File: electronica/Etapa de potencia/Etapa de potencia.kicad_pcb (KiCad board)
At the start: 2 copper layers, 70 x 45 mm, 23 parts, among them J1 Bornera Resorte, J2 Bornera Resorte, J3 Bornera Resorte, J4 Bornera 4 pines, J5 Header, Q1 MMBT2222, Q2 MMBT2222, Q3 MMBT2222, U1 ATmega328-PU, U2 ULN2003, U3 ULN2003, U4 MOC3031M, Y1 Crystal

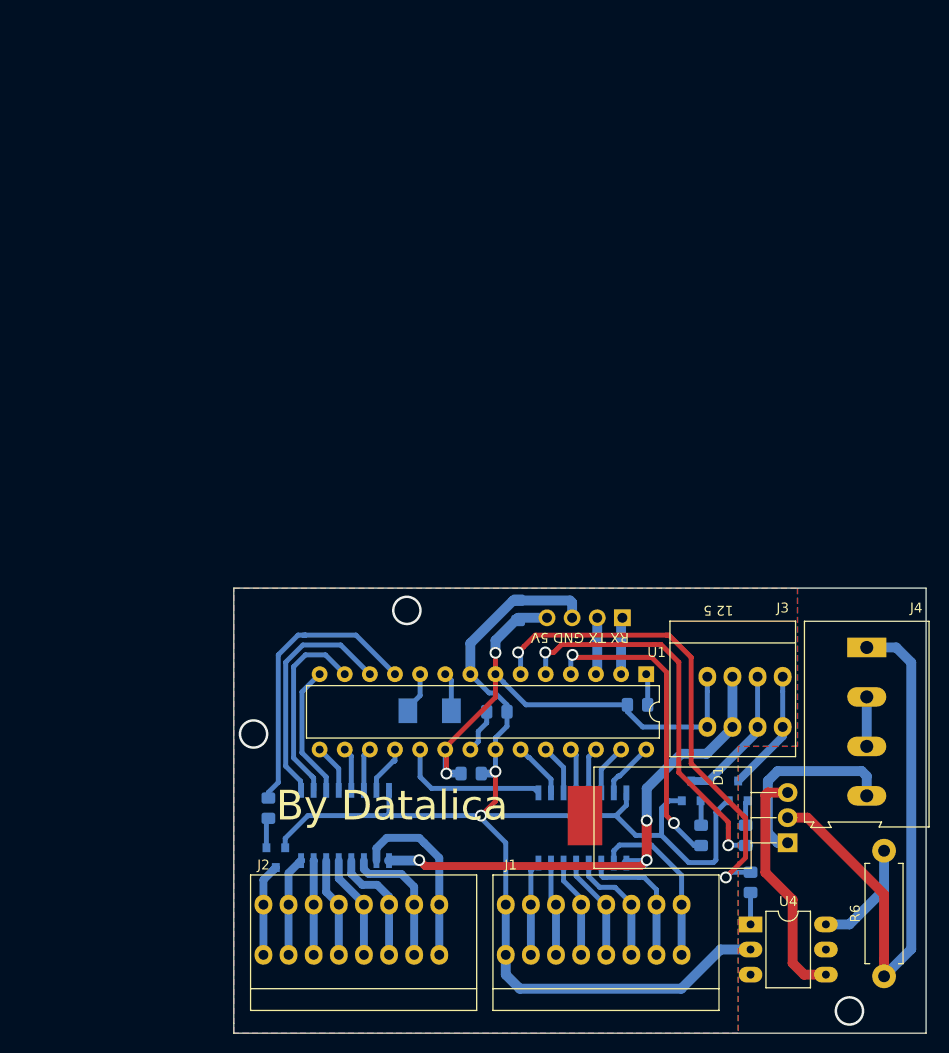
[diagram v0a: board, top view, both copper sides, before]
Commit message: ending first pcb
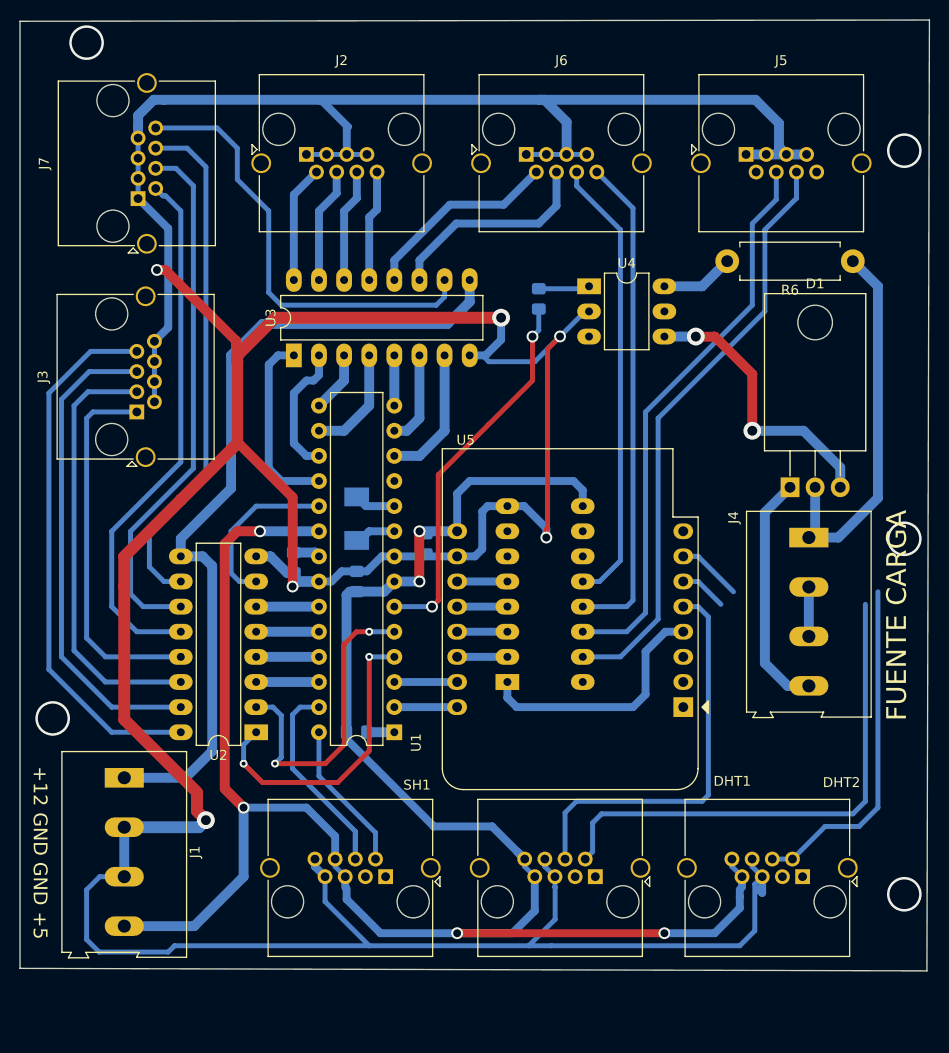
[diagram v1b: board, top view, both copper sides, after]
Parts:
- removed Q1, Q2, Q3: MMBT2222, Package_TO_SOT_SMD:SOT-23
- removed R3, R4, R5: 1K, Resistor_SMD:R_0805_2012Metric_Pad1.15x1.40mm_HandSolder
- added DHT1: RJ45, Connector_RJ:RJ45_Amphenol_RJHSE5380, F.Cu at (122.6, 130.2)
- added DHT2: RJ45, Connector_RJ:RJ45_Amphenol_RJHSE5380, F.Cu at (143.5, 130.2)
- added J6: RJ45, Connector_RJ:RJ45_Amphenol_RJHSE5380, F.Cu at (115.6, 57.1)
- added J7: RJ45, Connector_RJ:RJ45_Amphenol_RJHSE5380, F.Cu at (76.3, 61.6)
- added SH1: RJ45, Connector_RJ:RJ45_Amphenol_RJHSE5380, F.Cu at (101.3, 130.2)
- added U5: WeMos_D1_mini, Module:WEMOS_D1_mini_light, F.Cu at (131.4, 113.0)
- added U6: ULN2002A, Package_DIP:DIP-16_W7.62mm_LongPads, B.Cu at (113.7, 110.5)
- J1: value Bornera Resorte -> Bornera 4 pines; footprint potenciaFootprints:BorneraKF141R_8Pins -> TerminalBlock:TerminalBlock_Altech_AK300-4_P5.00mm
- J2: value Bornera Resorte -> RJ45; footprint potenciaFootprints:BorneraKF141R_8Pins -> Connector_RJ:RJ45_Amphenol_RJHSE5380
- J3: value Bornera Resorte -> RJ45; footprint potenciaFootprints:BorneraKF141R_4Pins -> Connector_RJ:RJ45_Amphenol_RJHSE5380
- J5: value Header -> RJ45; footprint Connector_PinHeader_2.54mm:PinHeader_1x04_P2.54mm_Vertical -> Connector_RJ:RJ45_Amphenol_RJHSE5380; moved to F.Cu
- U2, U3: footprint Package_SO:SOIC-16W_5.3x10.2mm_P1.27mm -> Package_DIP:DIP-16_W7.62mm_LongPads; moved to F.Cu
- moved J3 74.0 mm to (76.2, 83.2), turned to 90 degrees
- moved J2 73.0 mm to (93.3, 57.1)
- moved R6 72.4 mm to (148.6, 67.9), turned to 180 degrees
- moved U4 66.5 mm to (121.9, 70.5)
- moved R2 62.8 mm to (116.8, 71.8), turned to 270 degrees
- moved J5 48.5 mm to (137.8, 57.1), turned to 0 degrees
- moved U3 47.8 mm to (92.1, 77.5), turned to 90 degrees
- moved J1 39.8 mm to (74.9, 120.2), turned to 270 degrees
- moved D1 35.9 mm to (142.2, 90.8), turned to 0 degrees
- moved U2 34.4 mm to (88.3, 115.6), turned to 180 degrees
- moved R1 28.5 mm to (98.4, 115.6)
- moved U1 26.1 mm to (102.2, 115.6), turned to 180 degrees
- moved C1 25.5 mm to (92.1, 98.4), turned to 270 degrees
- moved C3 23.7 mm to (105.4, 96.5), turned to 270 degrees
- moved Y1 20.8 mm to (98.4, 94.0), turned to 90 degrees
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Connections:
- J1 pad 1: GND -> +12V
- J1 pad 2: VO1 -> GND
- J1 pad 3: VO2 -> GND
- J1 pad 4: VO3 -> +5V
- J2 pad 1: L05 -> GND
- J2 pad 3: LO3 -> GND
- J2 pad 4: LO2 -> LO3
- J2 pad 5: LO1 -> GND
- J2 pad 6: VO10 -> LO2
- J2 pad 7: VO9 -> GND
- J2 pad 8: VO8 -> LO1
- J3 pad 1: MO1 -> VO1
- J3 pad 2: MO2 -> GND
- J3 pad 3: +12V -> VO2
- J3 pad 4: +5V -> GND
- J5 pad 1: RX -> GND
- J5 pad 2: TX -> HO1
- J5 pad 4: +5V -> PSHO2
- U1 pad 11: L5 -> Net-(U1-Pad11)
- U1 pad 27: V2 -> SH_I1
- U1 pad 28: V1 -> SH_I2
- U1 pad 4: M2 -> V2
- U1 pad 5: M1 -> V1
- U2 pad 1: V7 -> V2
- U2 pad 13: VO4 -> VO1
- U2 pad 14: VO3 -> VO2
- U2 pad 15: VO2 -> VO3
- U2 pad 16: VO1 -> VO4
- U2 pad 2: V6 -> V1
- U2 pad 3: V5 -> V3
- U2 pad 5: V3 -> V5
- U2 pad 6: V2 -> V6
- U2 pad 7: V1 -> V7
- U3 pad 1: L4 -> V8
- U3 pad 2: L3 -> V9
- U3 pad 3: L2 -> L1
- U3 pad 4: L1 -> V10
- U3 pad 5: V10 -> L2
- U3 pad 6: V9 -> L3
- U3 pad 7: V8 -> L4
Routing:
- net GND: track 145.8 -> 456.8 mm, vias 2 -> 6
- net +5V: track 57.5 -> 212.6 mm, vias 2 -> 6
- net PSHO1: track 0.00 -> 60.2 mm
- net PSHO2: track 0.00 -> 57.2 mm
- net DHT_I2: track 0.00 -> 57.1 mm
- net VO4: track 10.7 -> 54.5 mm
- net VO5: track 12.0 -> 54.4 mm
- net DHT_I3: track 0.00 -> 41.2 mm
- net DHT_I1: track 0.00 -> 40.9 mm
- net VO6: track 14.0 -> 54.1 mm
- net VO3: track 10.0 -> 49.0 mm
- net MO1: track 12.4 -> 50.2 mm
- net VO7: track 17.7 -> 52.5 mm
- net M1: track 39.8 -> 5.08 mm, vias 2 -> 0
- net VO2: track 9.49 -> 43.8 mm
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- removed copper zone on B.Cu, net GND
- removed copper zone on F.Cu, net GND
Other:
- board size 70 x 45 mm -> 91.9 x 96.1 mm
- board text added: "+12 GND GND +5"
- board text added: "FUENTE CARGA"
- board text removed: "12 5"
- board text removed: "By Datalica"
- board text removed: "RX TX GND 5V"
